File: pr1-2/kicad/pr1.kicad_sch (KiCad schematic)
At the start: 8 parts, among them SW1 SW-SPDT, SW2 SW-SPDT, U1 STM32F103C8, U2 STM32F103C8

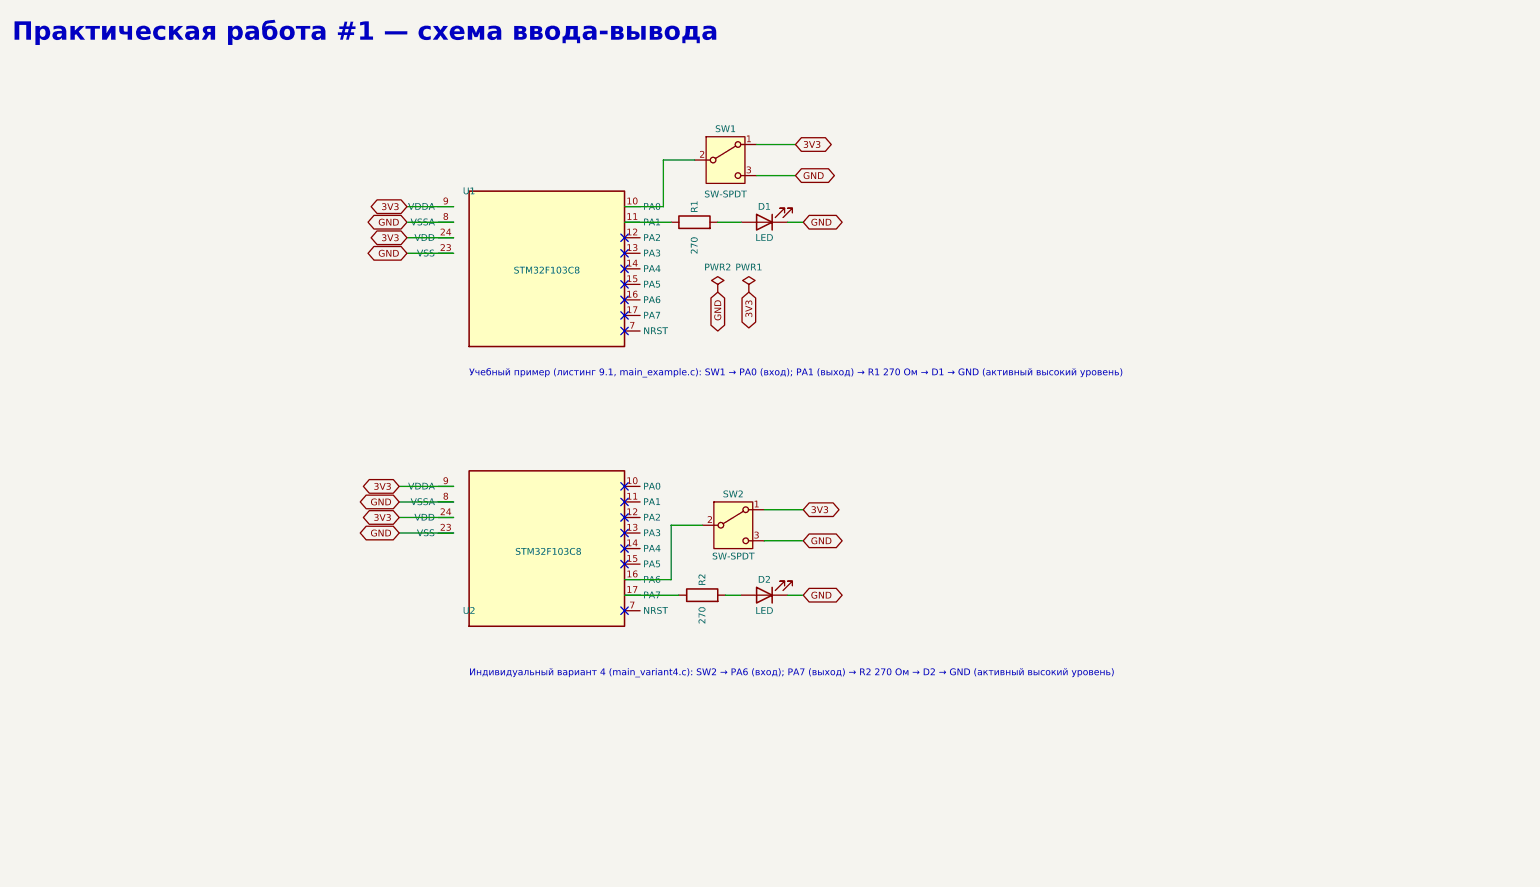
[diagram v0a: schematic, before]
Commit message: (fix): fix formatting; fix images
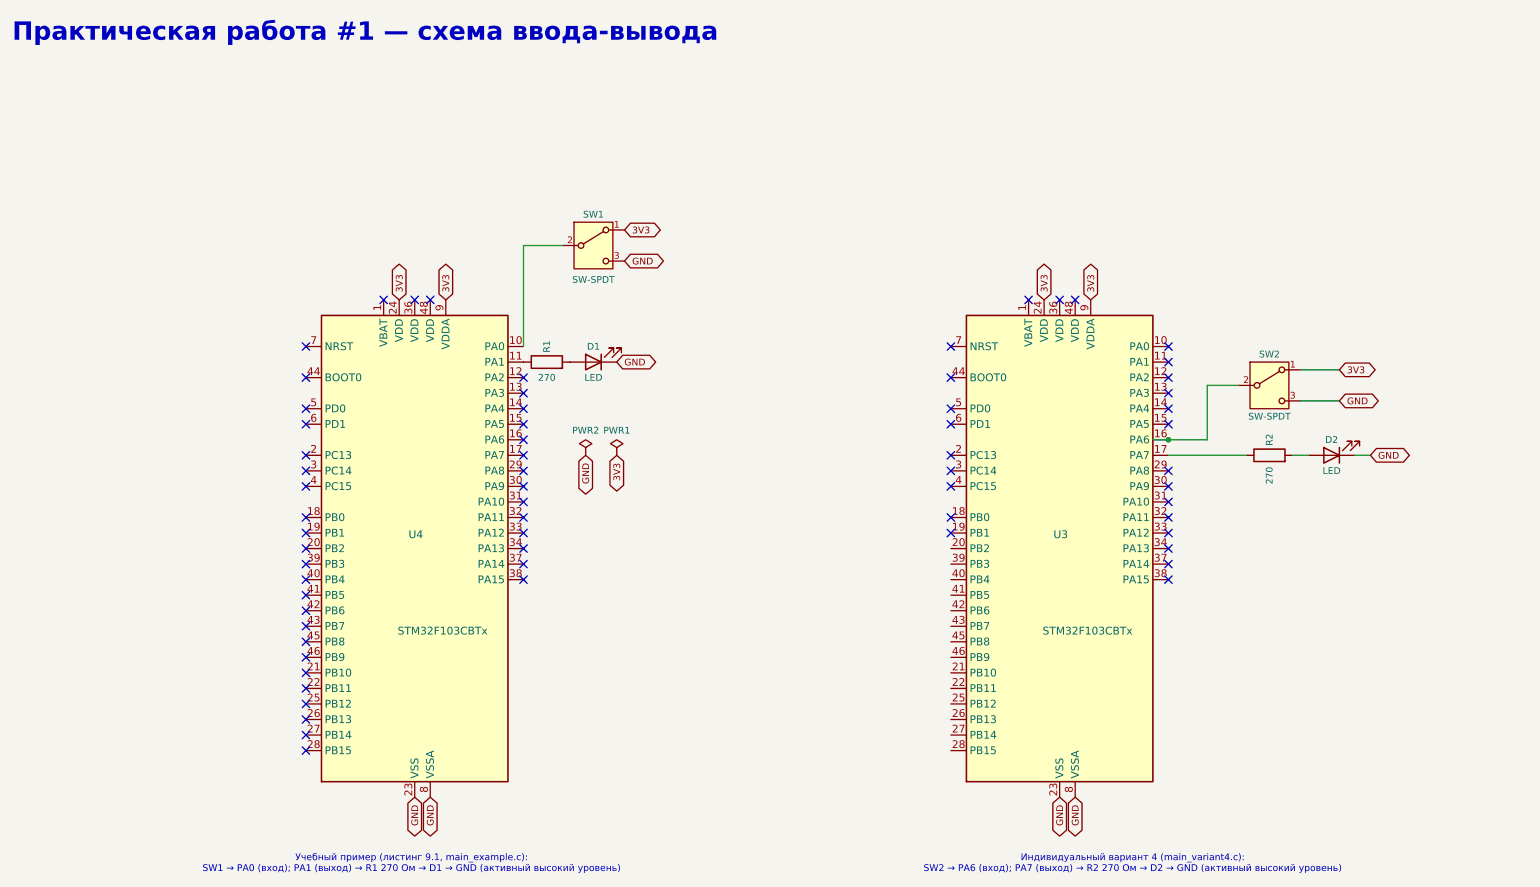
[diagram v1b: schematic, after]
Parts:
- removed U1, U2: STM32F103C8, symbol pr1:STM32F103C8
- added U3, U4: STM32F103CBTx, Package_QFP:LQFP-48_7x7mm_P0.5mm, symbol MCU_ST_STM32F1:STM32F103CBTx
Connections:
- net 3V3: now also U3.24 (VDD), U3.9 (VDDA), U4.24 (VDD), U4.9 (VDDA)
- net GND: now also U3.23 (VSS), U3.35 (VSS), U3.47 (VSS), U3.8 (VSSA), U4.23 (VSS), U4.35 (VSS), U4.47 (VSS), U4.8 (VSSA)
- net at SW1.2 (B): now also U4.10 (PA0)
- net at R1.1: now also U4.11 (PA1)
- net at SW2.2 (B): now also U3.16 (PA6)
- net at R2.1: now also U3.17 (PA7)
- no-connect marks 14 -> 66
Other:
- moved on the sheet: D1, D2, R1, R2, SW1, SW2
